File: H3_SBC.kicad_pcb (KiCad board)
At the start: 6 copper layers, 50 x 40 mm, 167 parts, among them CN1 YXT-BB10-50P-02, CN2 YXT-BB10-50P-02, CN3 YXT-BB10-50P-02, Q1 WPM1481-6/TR, U1 H3, U10 XT28EG32GA4YJECGA, U2 AXP223_C2997893, U5 AP2127K-2.5, U7 MT41K512M16VRP-107 IT:P, U9 RTL8211E-VB-CG, X1 X201232768KLD2SI, X2 SMD-5032_4P 24M 20pf, X3 5YAA25000121TF25E2

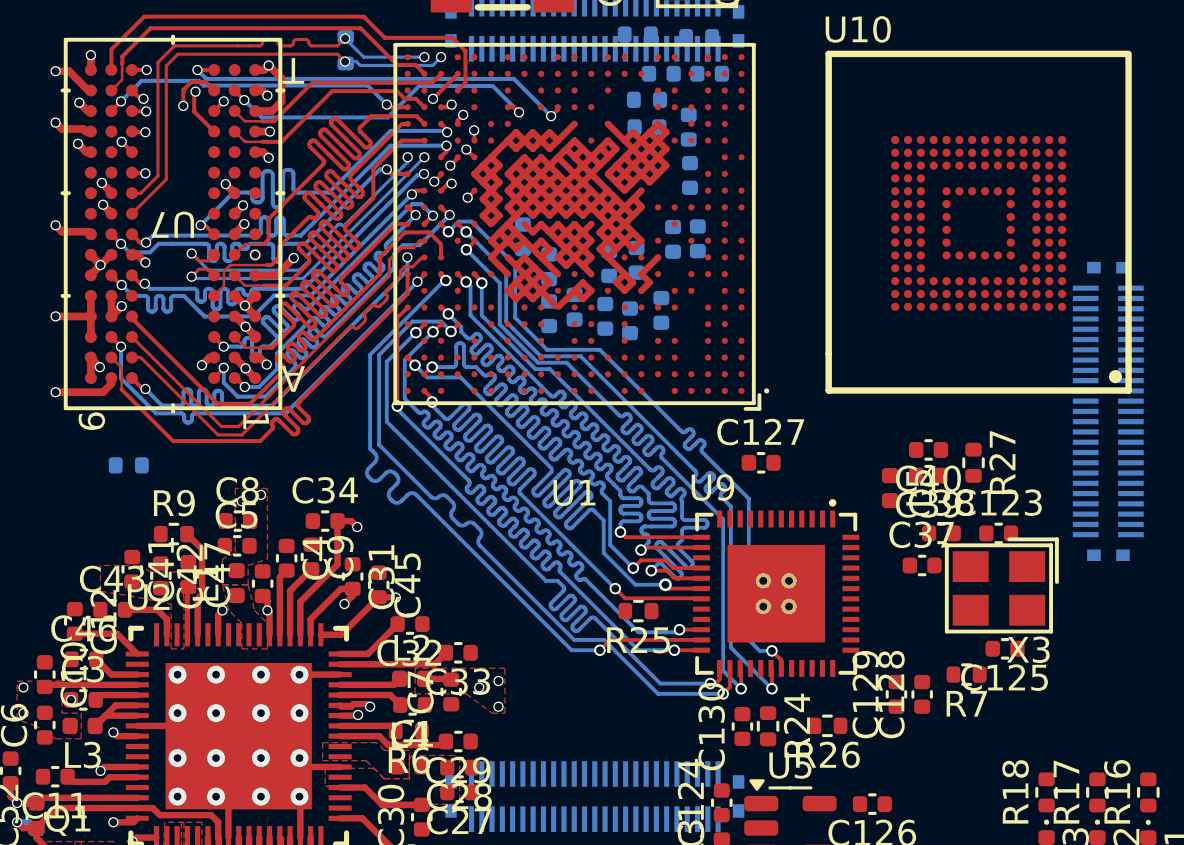
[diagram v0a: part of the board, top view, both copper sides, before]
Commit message: more tuning changes
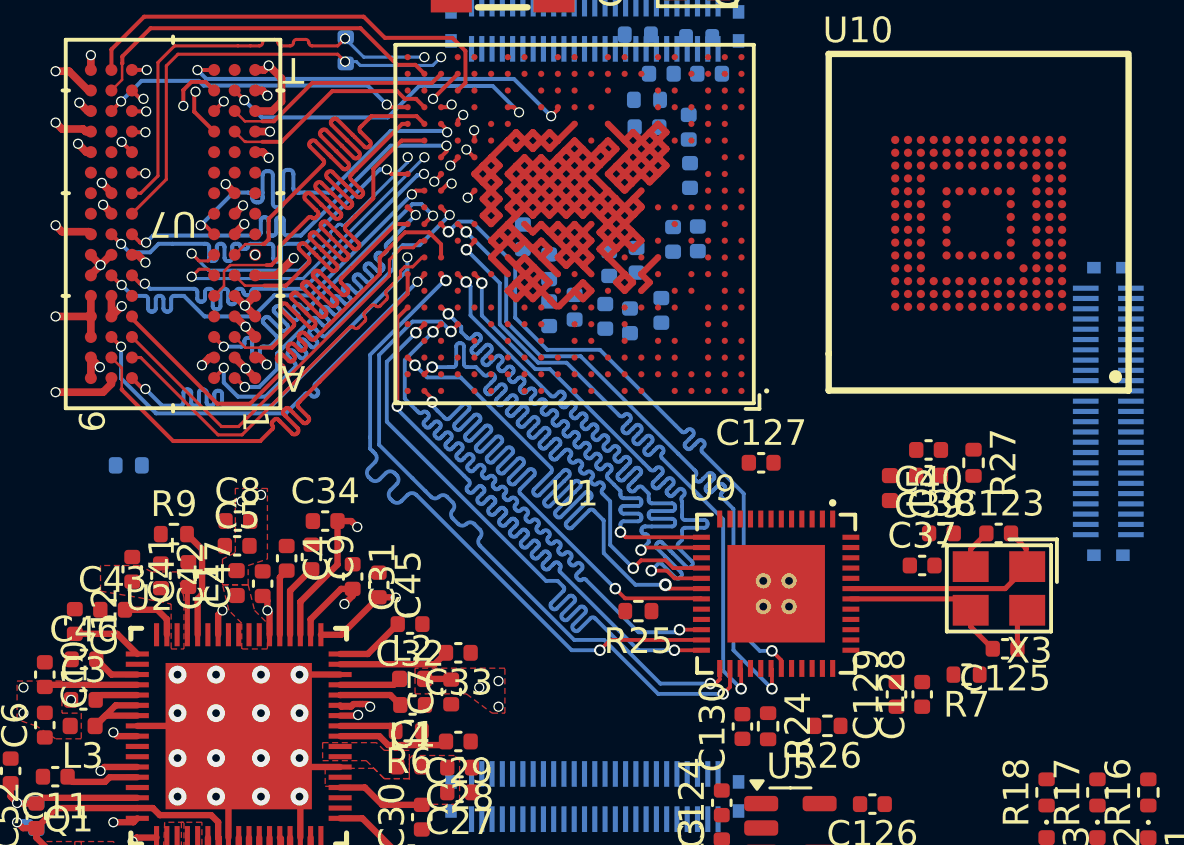
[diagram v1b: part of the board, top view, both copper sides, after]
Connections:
- U9 pad : GND -> (no net)
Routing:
- net /Ethernet/CKXTAL_IN: track 0.00 -> 8.78 mm
- net /Ethernet/CKXTAL_OUT: track 0.00 -> 6.71 mm
- net GND: track 103.9 -> 108.0 mm
